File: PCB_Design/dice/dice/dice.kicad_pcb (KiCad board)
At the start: 2 copper layers, 50 x 50 mm, 23 parts, among them J1 USB_C_Receptacle, SW1 SW_Push, U1 NE555D, U2 4017

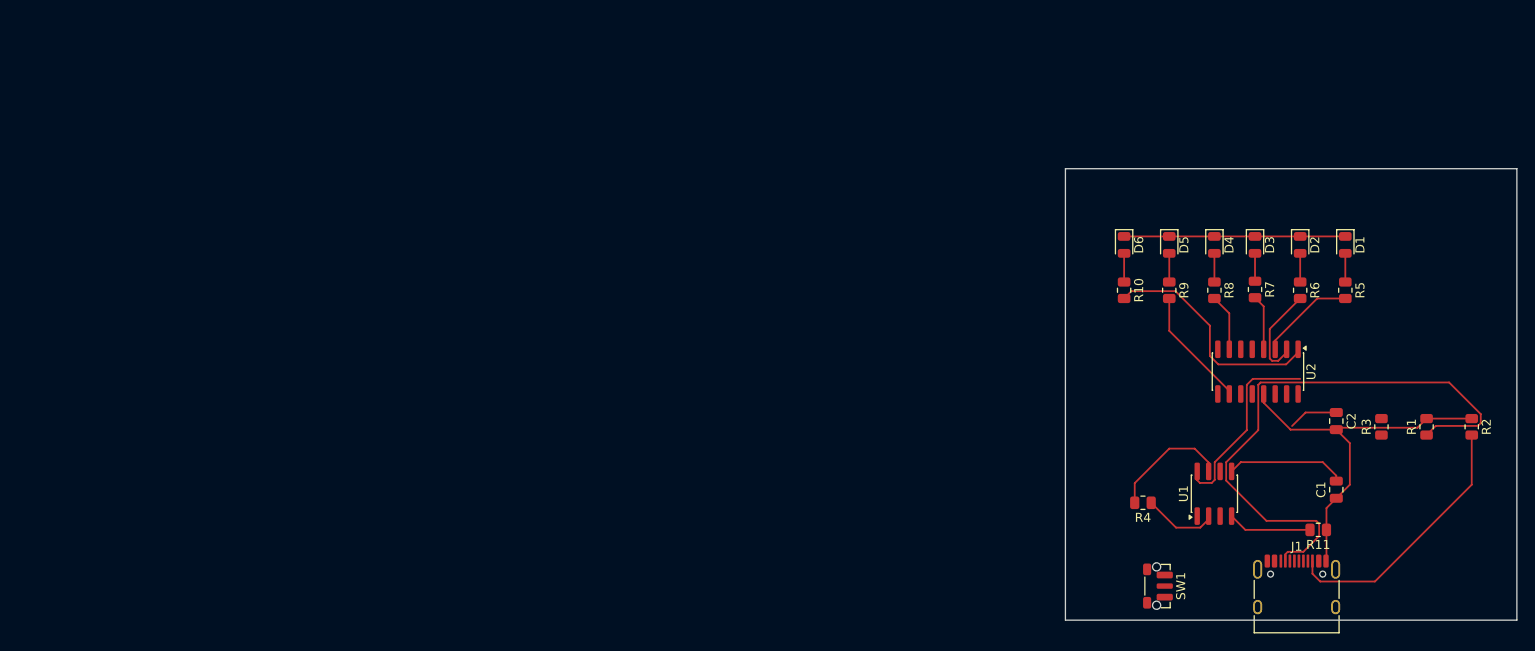
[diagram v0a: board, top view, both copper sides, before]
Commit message: backup pcb
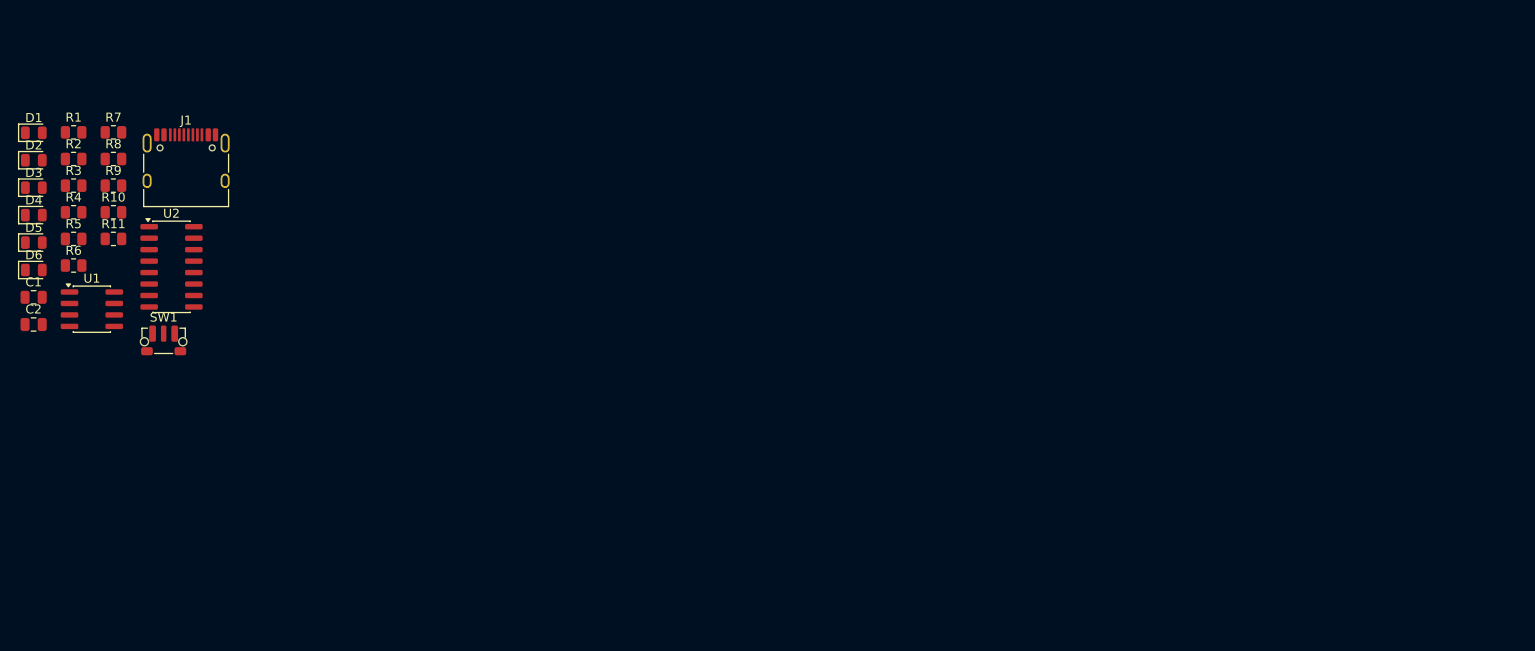
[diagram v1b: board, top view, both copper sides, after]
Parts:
- moved R2 157.7 mm to (56.2, 67.4), turned to 0 degrees
- moved R1 153.4 mm to (56.2, 64.5), turned to 0 degrees
- moved R3 147.3 mm to (56.2, 70.4), turned to 0 degrees
- moved C1 145.8 mm to (51.7, 82.7), turned to 0 degrees
- moved D1 145.8 mm to (51.7, 64.5), turned to 0 degrees
- moved C2 144.7 mm to (51.7, 85.8), turned to 0 degrees
- moved R5 141.0 mm to (56.2, 76.3), turned to 0 degrees
- moved D2 140.6 mm to (51.7, 67.6), turned to 0 degrees
- moved R11 137.3 mm to (60.6, 76.3), turned to 0 degrees
- moved R6 135.9 mm to (56.2, 79.2), turned to 0 degrees
- moved D3 135.4 mm to (51.7, 70.6), turned to 0 degrees
- moved J1 131.7 mm to (68.6, 68.8)
- moved D4 130.8 mm to (51.7, 73.6), turned to 0 degrees
- moved R7 127.6 mm to (60.6, 64.5), turned to 0 degrees
- moved U1 126.0 mm to (58.2, 84.1), turned to 0 degrees
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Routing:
- net GND: track 66.5 -> 0.00 mm
- net Net-(J1-CC1): track 64.8 -> 0.00 mm
- net Net-(J1-CC2): track 29.3 -> 0.00 mm
- net Net-(U2-Q5): track 25.8 -> 0.00 mm
- net Net-(U1-VCC): track 21.4 -> 0.00 mm
- net Net-(U1-THRES): track 13.8 -> 0.00 mm
- net Net-(U1-DISCH): track 13.6 -> 0.00 mm
- net Net-(U2-Q4): track 13.3 -> 0.00 mm
- net Net-(U1-CONT): track 13.2 -> 0.00 mm
- net Net-(U2-Q1): track 10.7 -> 0.00 mm
- net Net-(U2-Q0): track 10.7 -> 0.00 mm
- net Net-(U1-~{RST}): track 9.31 -> 0.00 mm
- net Net-(U2-Q3): track 6.31 -> 0.00 mm
- net Net-(U2-Q2): track 6.11 -> 0.00 mm
- net Net-(D6-A): track 3.17 -> 0.00 mm
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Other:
- board outline removed

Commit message: usb led pcb
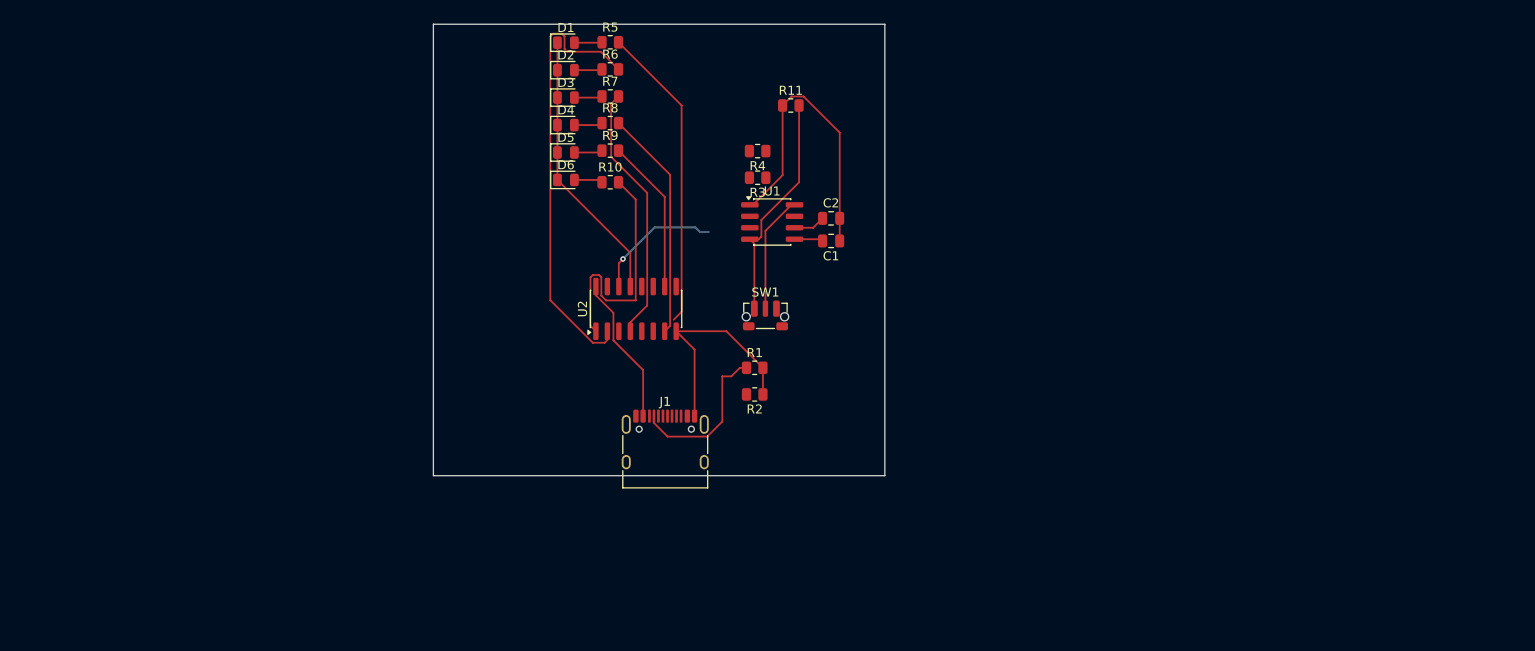
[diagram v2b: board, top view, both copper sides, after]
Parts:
- moved C2 89.1 mm to (140.1, 74.0)
- moved C1 88.5 mm to (140.1, 76.5), turned to 180 degrees
- moved R1 79.8 mm to (131.6, 90.5)
- moved R2 79.8 mm to (131.6, 93.5), turned to 180 degrees
- moved R11 76.5 mm to (135.6, 61.5)
- moved R4 76.1 mm to (131.9, 66.5), turned to 180 degrees
- moved U1 76.0 mm to (133.5, 74.4)
- moved R3 75.8 mm to (131.9, 69.5), turned to 180 degrees
- moved SW1 66.7 mm to (132.8, 84.9)
- moved R5 63.3 mm to (115.6, 54.5)
- moved R6 63.3 mm to (115.6, 57.5)
- moved J1 61.5 mm to (121.7, 100.0)
- moved D1 59.8 mm to (110.7, 54.5)
- moved D2 59.8 mm to (110.7, 57.6)
- moved D3 59.8 mm to (110.7, 60.6)
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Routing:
- net GND: track 0.00 -> 87.9 mm
- net Net-(U2-Q1): track 0.00 -> 48.7 mm
- net Net-(U2-Q0): track 0.00 -> 34.2 mm
- net Net-(U1-VCC): track 0.00 -> 30.1 mm
- net Net-(U2-Q2): track 0.00 -> 28.8 mm
- net Net-(U2-Q5): track 0.00 -> 27.6 mm
- net Net-(U2-Q3): track 0.00 -> 25.7 mm
- net Net-(U1-~{RST}): track 0.00 -> 25.5 mm
- net Net-(J1-CC1): track 0.00 -> 17.7 mm
- net Net-(U2-Q4): track 0.00 -> 17.2 mm
- net Net-(U1-OUT): track 0.00 -> 14.4 mm, vias 0 -> 1
- net Net-(D6-A): track 0.00 -> 3.65 mm
- net Net-(U1-THRES): track 0.00 -> 3.53 mm
- net Net-(U1-CONT): track 0.00 -> 3.18 mm
- net Net-(D4-A): track 0.00 -> 3.15 mm
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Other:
- board outline added: 50 x 50 mm
